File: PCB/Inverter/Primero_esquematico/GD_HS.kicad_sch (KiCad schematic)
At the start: 46 parts, among them T7 750317595, U40 LM25180QNGURQ1, U41 UCC21750QDWRQ1, U42 LP2951-5.0_VSSOP

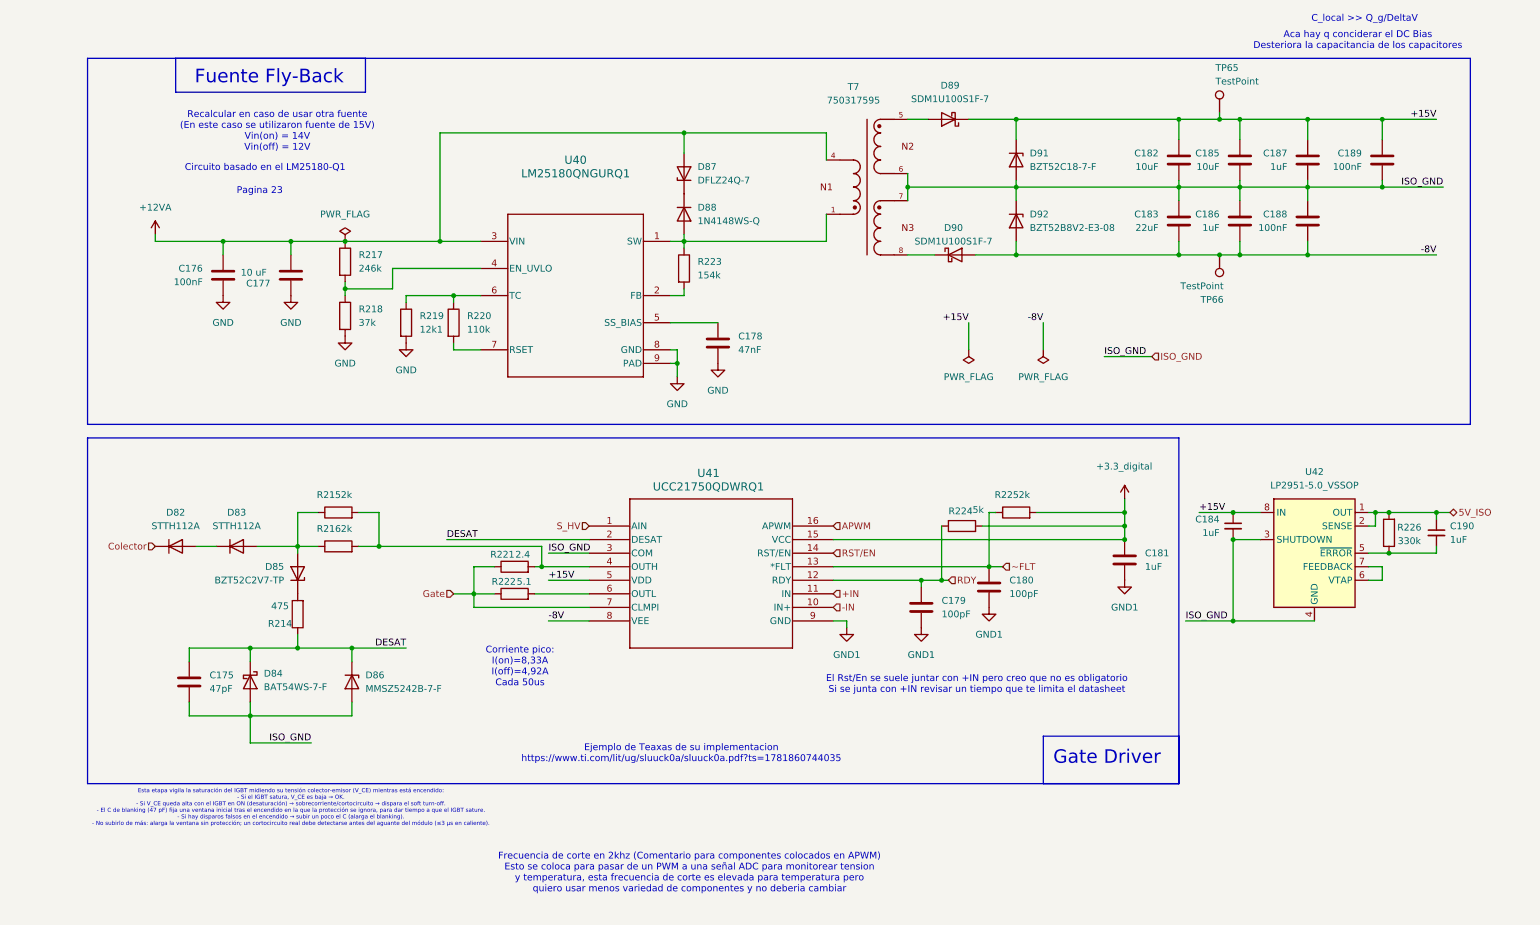
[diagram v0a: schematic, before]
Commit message: Corregi cosas de la placa
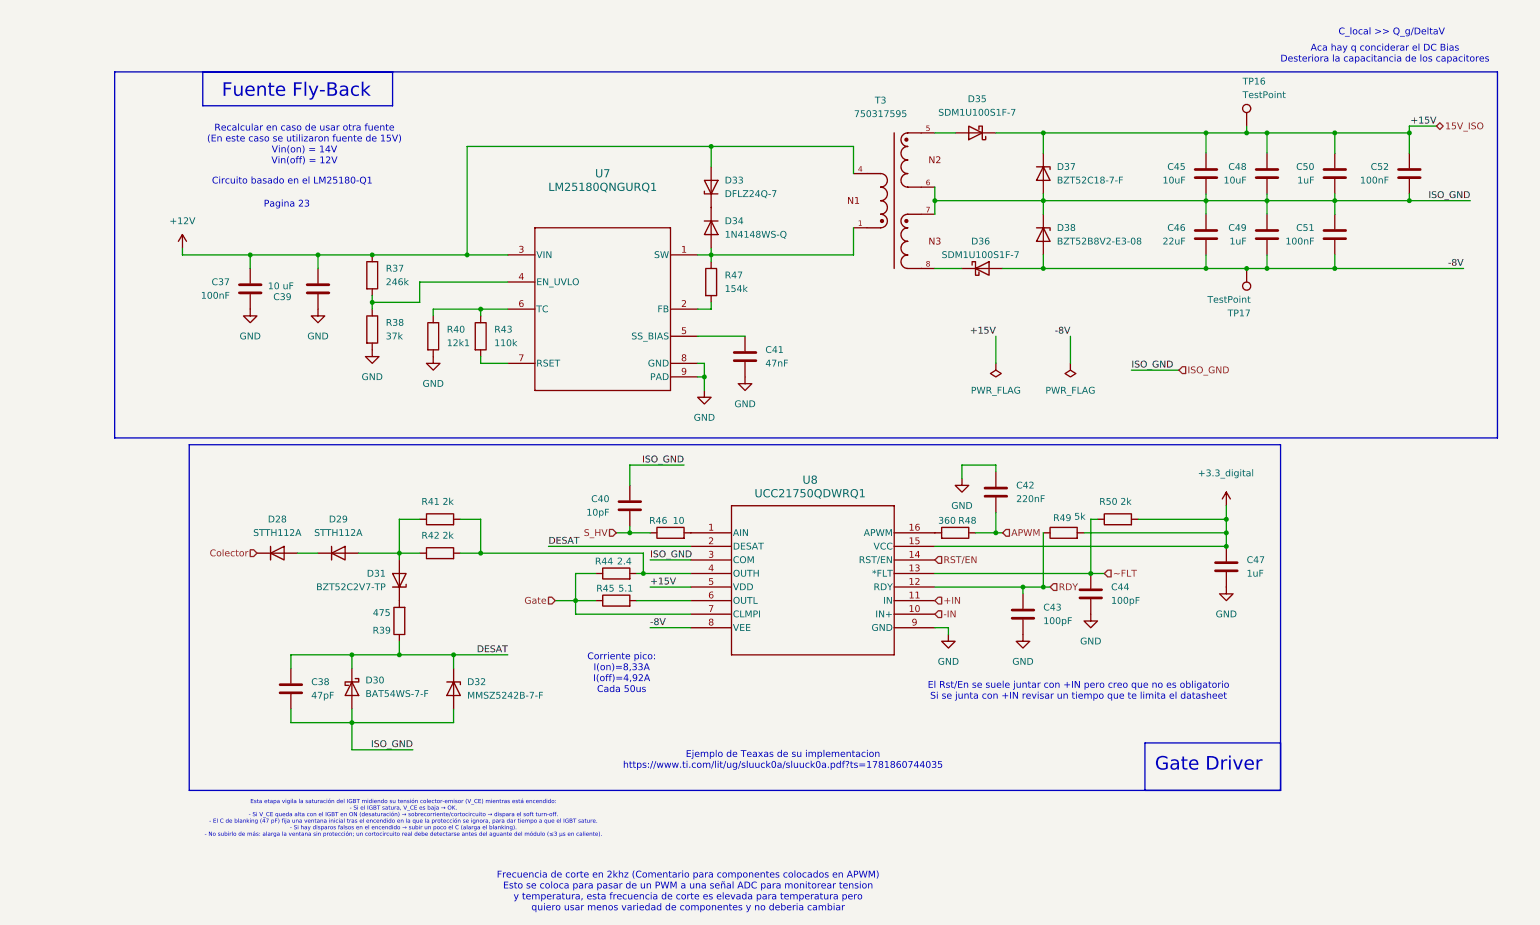
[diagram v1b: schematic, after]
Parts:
- removed C175: 47pF, Capacitor_SMD:C_0603_1608Metric_Pad1.08x0.95mm_HandSolder, symbol Device:C
- removed C176, C188, C189: 100nF, Capacitor_SMD:C_0402_1005Metric, symbol Device:C
- removed C177: 10 uF, Capacitor_SMD:C_1206_3216Metric, symbol Device:C
- removed C178: 47nF, Capacitor_SMD:C_0402_1005Metric_Pad0.74x0.62mm_HandSolder, symbol Device:C
- removed C179, C180: 100pF, Capacitor_SMD:C_0402_1005Metric, symbol Device:C
- removed C181: 1uF, Capacitor_SMD:C_0603_1608Metric, symbol Device:C
- removed C182, C185: 10uF, Capacitor_SMD:C_1210_3225Metric, symbol Device:C
- removed C183: 22uF, Capacitor_SMD:C_1210_3225Metric, symbol Device:C
- removed C184, C190: 1uF, Capacitor_SMD:C_0603_1608Metric, symbol Device:C_Small
- removed C186, C187: 1uF, Capacitor_SMD:C_0805_2012Metric, symbol Device:C
- removed D82, D83: STTH112A, Diode_SMD:D_SOD-323F, symbol Device:D
- removed D84: BAT54WS-7-F, Diode_SMD:D_SOD-323_HandSoldering, symbol Device:D_Schottky
- removed D85: BZT52C2V7-TP, Diode_SMD:D_SOD-123, symbol Device:D_Zener
- removed D86: MMSZ5242B-7-F, Diode_SMD:D_SOD-123, symbol Device:D_Zener
- removed D87: DFLZ24Q-7, Diode_SMD:D_PowerDI-123, symbol Device:D_Zener
- removed D88: 1N4148WS-Q, Diode_SMD:D_SOD-323F, symbol Device:D
- removed D89, D90: SDM1U100S1F-7, Diode_SMD:D_SOD-123F, symbol Device:D_Schottky
- removed D91: BZT52C18-7-F, Diode_SMD:D_SOD-123, symbol Device:D_Zener
- removed D92: BZT52B8V2-E3-08, Diode_SMD:D_SOD-123, symbol Device:D_Zener
- removed R214: 475, Resistor_SMD:R_0805_2012Metric, symbol Device:R
- removed R215, R216: 2k, Resistor_SMD:R_0805_2012Metric, symbol Device:R
- removed R217: 246k, Resistor_SMD:R_0402_1005Metric, symbol Device:R
- removed R218: 37k, Resistor_SMD:R_0402_1005Metric, symbol Device:R
- removed R219: 12k1, Resistor_SMD:R_0402_1005Metric, symbol Device:R
- removed R220: 110k, Resistor_SMD:R_0402_1005Metric, symbol Device:R
- removed R221: 2.4, Resistor_SMD:R_1206_3216Metric, symbol Device:R
- removed R222: 5.1, Resistor_SMD:R_1206_3216Metric, symbol Device:R
- removed R223: 154k, Resistor_SMD:R_0402_1005Metric_Pad0.72x0.64mm_HandSolder, symbol Device:R
- removed R224: 5k, Resistor_SMD:R_0402_1005Metric, symbol Device:R
- removed R225: 2k, Resistor_SMD:R_0402_1005Metric, symbol Device:R
- removed R226: 330k, Resistor_SMD:R_0402_1005Metric, symbol Device:R
- removed T7: 750317595, Snapeda:WE-FLYTI_EP7_4436, symbol Snapeda:750317595
- removed TP65, TP66: TestPoint, TestPoint:TestPoint_Pad_D1.0mm, symbol Connector:TestPoint
- removed U40: LM25180QNGURQ1, Snapeda:NGU0008C, symbol Snapeda:LM25180QNGURQ1
- removed U41: UCC21750QDWRQ1, Snapeda:SOIC16_DW_TEX-L, symbol Snapeda:UCC21750QDWRQ1
- removed U42: LP2951-5.0_VSSOP, Package_SO:VSSOP-8_3x3mm_P0.65mm, symbol Regulator_Linear:LP2951-5.0_VSSOP
- added C37, C51, C52: 100nF, Capacitor_SMD:C_0402_1005Metric, symbol Device:C
- added C38: 47pF, Capacitor_SMD:C_0603_1608Metric_Pad1.08x0.95mm_HandSolder, symbol Device:C
- added C39: 10 uF, Capacitor_SMD:C_1206_3216Metric, symbol Device:C
- added C40: 10pF, Capacitor_SMD:C_0402_1005Metric, symbol Device:C
- added C41: 47nF, Capacitor_SMD:C_0402_1005Metric_Pad0.74x0.62mm_HandSolder, symbol Device:C
- added C42: 220nF, Capacitor_SMD:C_0402_1005Metric, symbol Device:C
- added C43, C44: 100pF, Capacitor_SMD:C_0402_1005Metric, symbol Device:C
- added C45, C48: 10uF, Capacitor_SMD:C_1210_3225Metric, symbol Device:C
- added C46: 22uF, Capacitor_SMD:C_1210_3225Metric, symbol Device:C
- added C47: 1uF, Capacitor_SMD:C_0603_1608Metric, symbol Device:C
- added C49, C50: 1uF, Capacitor_SMD:C_0805_2012Metric, symbol Device:C
- added D28, D29: STTH112A, Diode_SMD:D_SOD-323F, symbol Device:D
- added D30: BAT54WS-7-F, Diode_SMD:D_SOD-323_HandSoldering, symbol Device:D_Schottky
- added D31: BZT52C2V7-TP, Diode_SMD:D_SOD-123, symbol Device:D_Zener
- added D32: MMSZ5242B-7-F, Diode_SMD:D_SOD-123, symbol Device:D_Zener
- added D33: DFLZ24Q-7, Diode_SMD:D_PowerDI-123, symbol Device:D_Zener
- added D34: 1N4148WS-Q, Diode_SMD:D_SOD-323F, symbol Device:D
- added D35, D36: SDM1U100S1F-7, Diode_SMD:D_SOD-123F, symbol Device:D_Schottky
- added D37: BZT52C18-7-F, Diode_SMD:D_SOD-123, symbol Device:D_Zener
- added D38: BZT52B8V2-E3-08, Diode_SMD:D_SOD-123, symbol Device:D_Zener
- added R37: 246k, Resistor_SMD:R_0402_1005Metric, symbol Device:R
- added R38: 37k, Resistor_SMD:R_0402_1005Metric, symbol Device:R
- added R39: 475, Resistor_SMD:R_0805_2012Metric, symbol Device:R
- added R40: 12k1, Resistor_SMD:R_0402_1005Metric, symbol Device:R
- added R41, R42: 2k, Resistor_SMD:R_0805_2012Metric, symbol Device:R
- added R43: 110k, Resistor_SMD:R_0402_1005Metric, symbol Device:R
- added R44: 2.4, Resistor_SMD:R_1206_3216Metric, symbol Device:R
- added R45: 5.1, Resistor_SMD:R_1206_3216Metric, symbol Device:R
- added R46: 10, Resistor_SMD:R_0402_1005Metric, symbol Device:R
- added R47: 154k, Resistor_SMD:R_0402_1005Metric_Pad0.72x0.64mm_HandSolder, symbol Device:R
- added R48: 360, Resistor_SMD:R_0402_1005Metric, symbol Device:R
- added R49: 5k, Resistor_SMD:R_0402_1005Metric, symbol Device:R
- added R50: 2k, Resistor_SMD:R_0402_1005Metric, symbol Device:R
- added T3: 750317595, Snapeda:WE-FLYTI_EP7_4436, symbol Snapeda:750317595
- added TP16, TP17: TestPoint, TestPoint:TestPoint_Pad_D1.0mm, symbol Connector:TestPoint
- added U7: LM25180QNGURQ1, Snapeda:NGU0008C, symbol Snapeda:LM25180QNGURQ1
- added U8: UCC21750QDWRQ1, Snapeda:SOIC16_DW_TEX-L, symbol Snapeda:UCC21750QDWRQ1
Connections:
- net +3.3_digital: now also C47.2, R49.2, R50.2, U8.15 (VCC)
- net +IN: now also U8.11 (IN)
- net -8V: now also C46.1, C49.1, C51.1, D36.2 (A), D38.2 (A), TP17.1, U8.8 (VEE)
- net -IN: now also U8.10 (IN+)
- net APWM: now also C42.1, R48.1
- net Colector: now also D28.1 (K)
- net DESAT: now also C38.2, D30.1 (K), D32.1 (K), R39.1, U8.2 (DESAT)
- net GND: now also C37.1, C39.2, C41.1, C42.2, C43.1, C44.1, C47.1, R38.2, R40.2, U7.8 (GND), U7.9 (PAD), U8.9 (GND)
- net Gate: now also R44.1, R45.1, U8.7 (CLMPI)
- net ISO_GND: now also C38.1, C40.2, C45.1, C46.2, C48.1, C49.2, C50.1, C51.2, C52.1, D30.2 (A), D32.2 (A), D37.2 (A), D38.1 (K), T3.6, T3.7, U8.3 (COM)
- net RDY: now also C43.2, R49.1, U8.12 (RDY)
- net RST/EN: now also U8.14 (RST/EN)
- net S_HV: now also C40.1, R46.1
- net ~FLT: now also C44.2, R50.1, U8.13 (*FLT)
- new net: R37.2, R38.1, U7.4 (EN_UVLO)
- new net: R45.2, U8.6 (OUTL)
- new net: R40.1, R43.1, U7.6 (TC)
- new net: R43.2, U7.7 (RSET)
- new net: D36.1 (K), T3.8
- new net: R46.2, U8.1 (AIN)
- new net: R48.2, U8.16 (APWM)
- new net: R41.2, R42.2, R44.2, U8.4 (OUTH)
- new net: D34.2 (A), R47.1, T3.1, U7.1 (SW)
- new net: D35.2 (A), T3.5
- new net: D29.2 (A), D31.2 (A), R41.1, R42.1
- new net: C41.2, U7.5 (SS_BIAS)
- new net: D33.1 (K), D34.1 (K)
- new net: D28.2 (A), D29.1 (K)
- new net: R47.2, U7.2 (FB)
- new net: D31.1 (K), R39.2
- new net +12V: C37.2, C39.1, D33.2 (A), R37.1, T3.4, U7.3 (VIN)
- new net 15V_ISO: C45.2, C48.2, C50.2, C52.2, D35.1 (K), D37.1 (K), TP16.1, U8.5 (VDD)
